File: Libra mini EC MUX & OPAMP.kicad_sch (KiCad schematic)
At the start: 16 parts, among them U6 OPA2365, U7 4052, U8 OPA2365, U9 4052

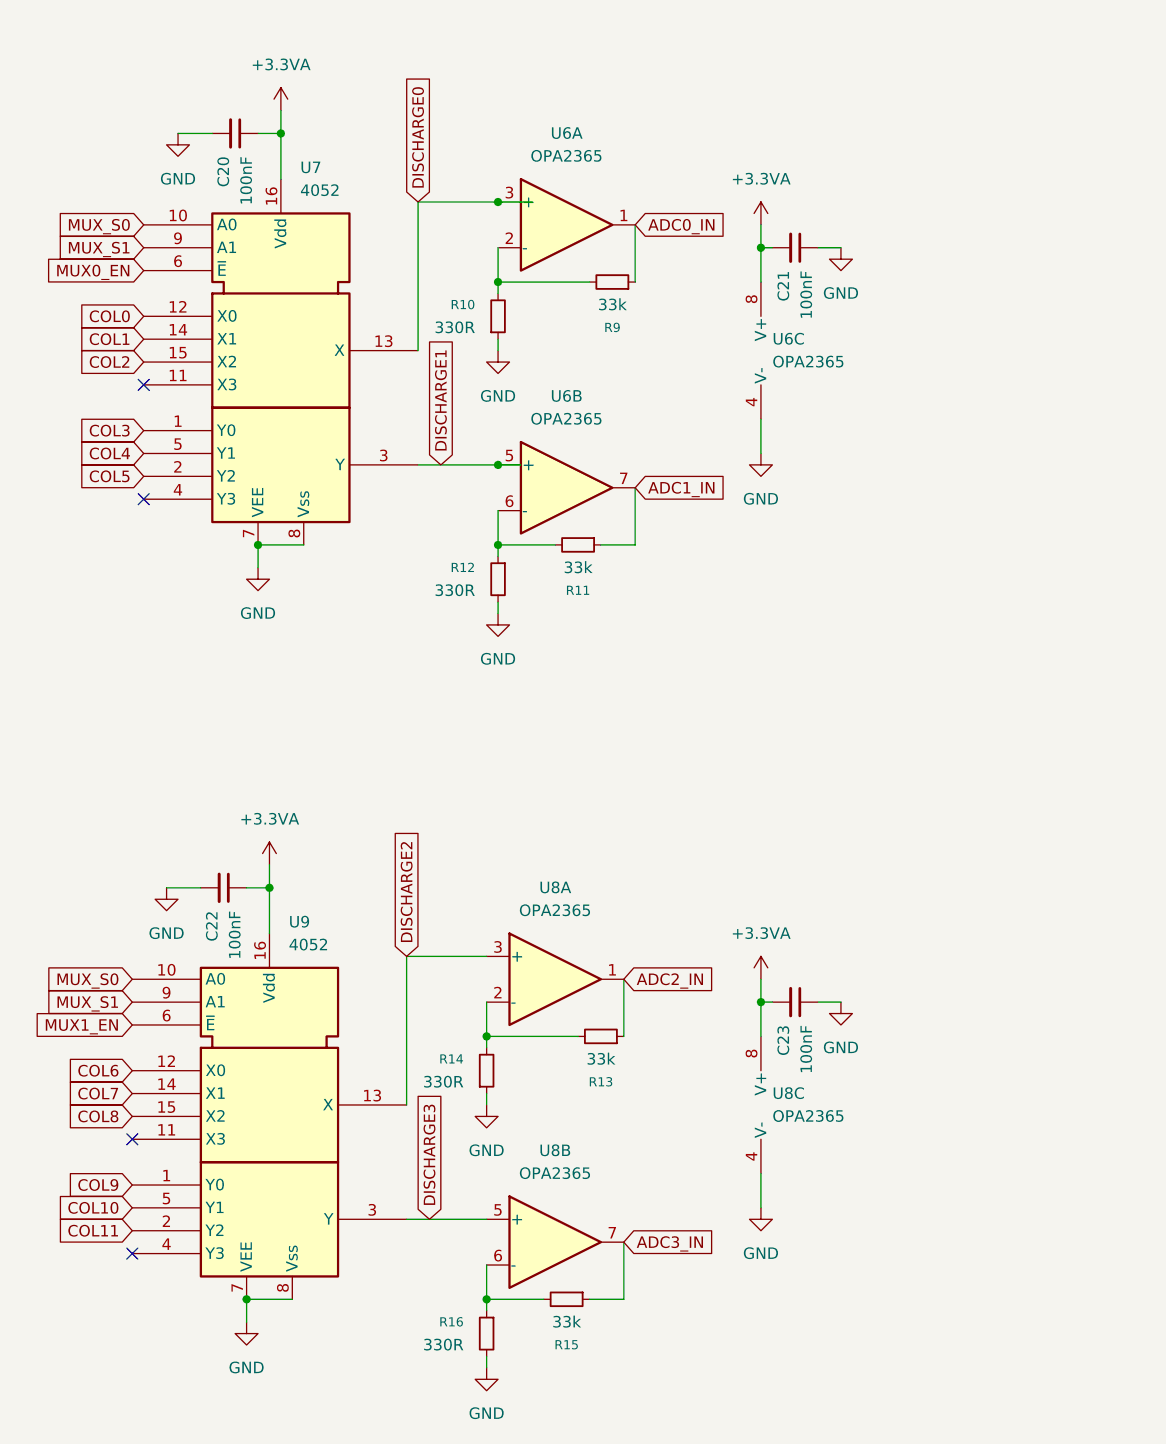
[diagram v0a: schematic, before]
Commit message: 13.04.2026
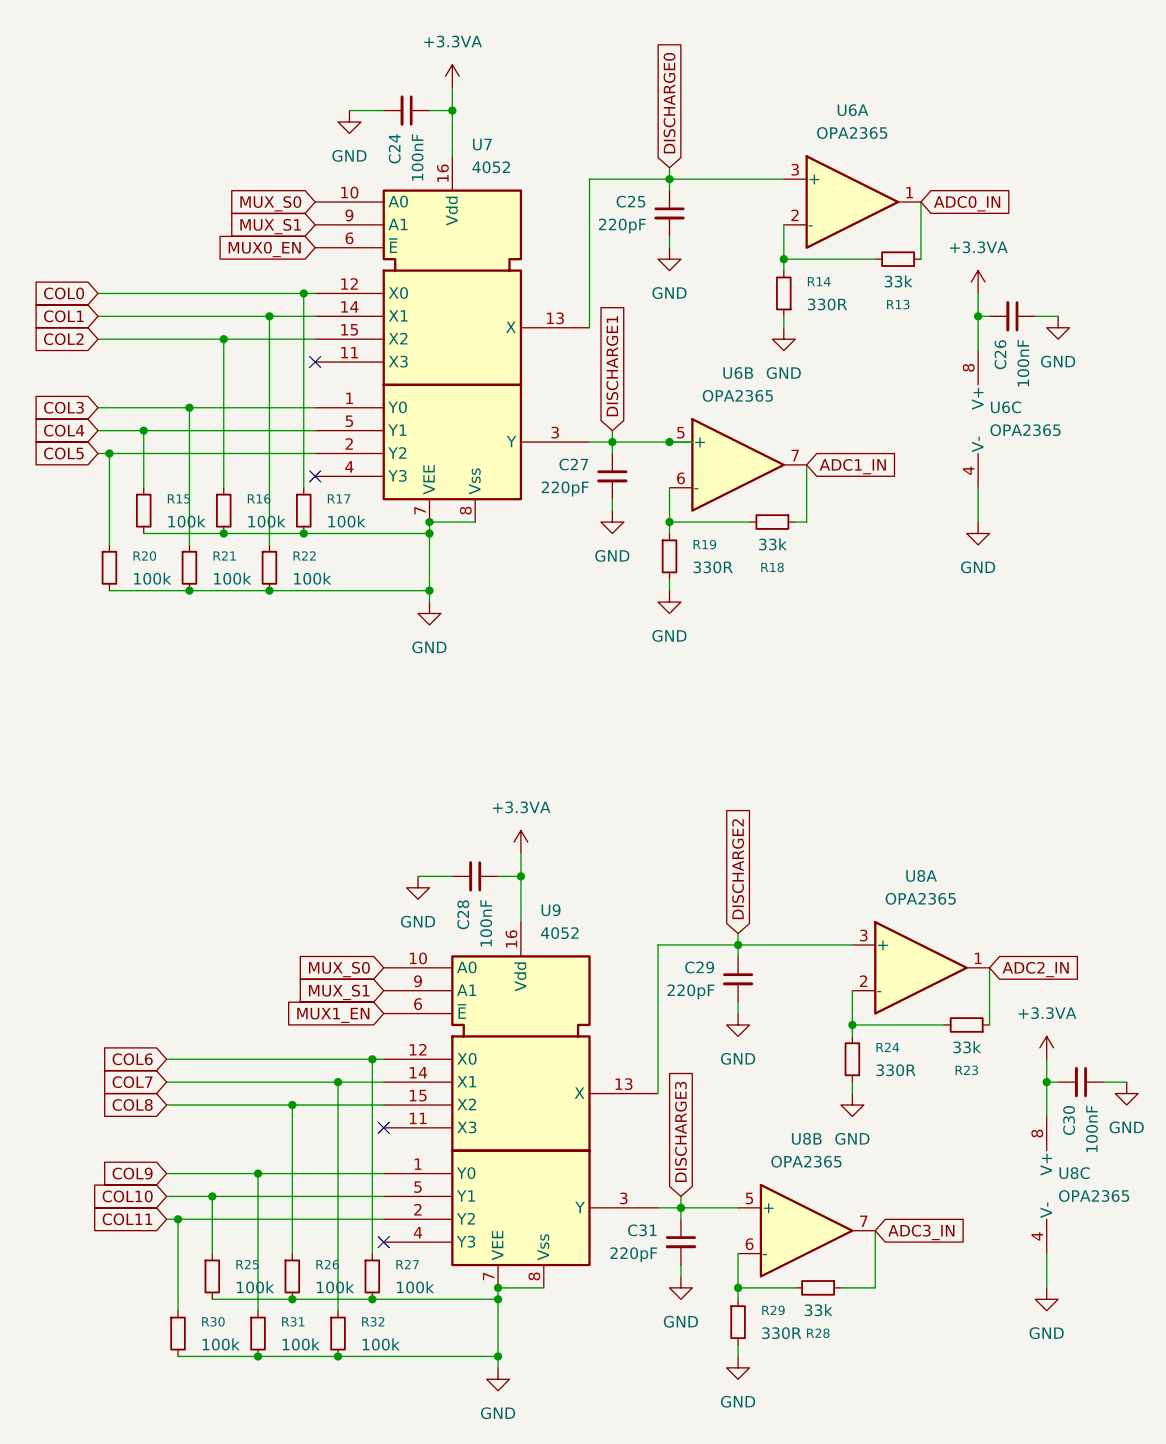
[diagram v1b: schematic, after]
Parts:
- added C25, C27, C29, C31: 220pF, Capacitor_SMD:C_0603_1608Metric, symbol Device:C_Small
- added R15, R16, R17, R20, R21, R22, R25, R26, R27, R30, R31, R32: 100k, Capacitor_SMD:C_0805_2012Metric, symbol Device:R_Small
- renumbered C20 to C24, C21 to C26, C22 to C28, C23 to C30, R9 to R13, R10 to R14, R11 to R18, R12 to R19, R13 to R23, R14 to R24, R15 to R28, R16 to R29
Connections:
- net COL0: now also R17.1
- net COL1: now also R22.1
- net COL10: now also R25.1
- net COL11: now also R30.1
- net COL2: now also R16.1
- net COL3: now also R21.1
- net COL4: now also R15.1
- net COL5: now also R20.1
- net COL6: now also R27.1
- net COL7: now also R32.1
- net COL8: now also R26.1
- net COL9: now also R31.1
- net DISCHARGE0: now also C25.1
- net DISCHARGE1: now also C27.1
- net DISCHARGE2: now also C29.1
- net DISCHARGE3: now also C31.1
- net GND: now also C25.2, C27.2, C29.2, C31.2, R15.2, R16.2, R17.2, R20.2, R21.2, R22.2, R25.2, R26.2, R27.2, R30.2, R31.2, R32.2
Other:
- moved on the sheet: C24, C26, C28, C30, R13, R14, R18, R19, R23, R24, R28, R29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
